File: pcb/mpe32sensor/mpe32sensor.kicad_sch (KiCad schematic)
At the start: 6 parts, among them J1 Conn_01x04, J2 Conn_01x01, J3 Conn_01x01, U1 TMAG5273

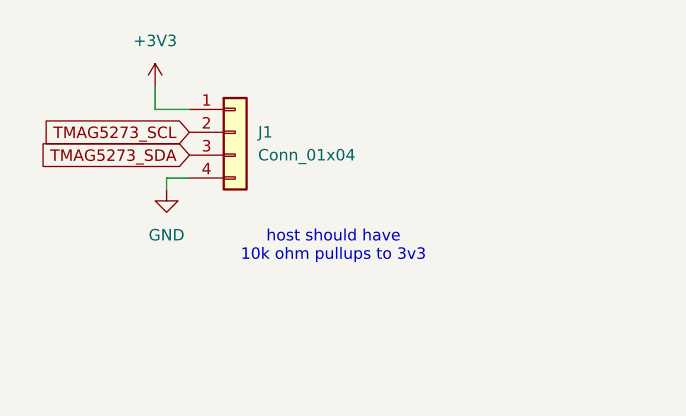
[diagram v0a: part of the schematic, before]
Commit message: production file changes + ide setup
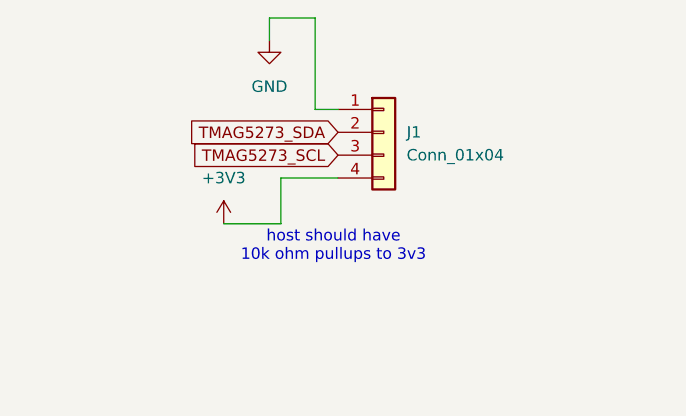
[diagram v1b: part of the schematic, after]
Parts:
- C1: MPN (none) -> 100nF 0603 X7R
- D1: MPN (none) -> SK6812MINI-E OPSCO Optoelectronics C5149201
- J1: MPN (none) -> SM04B-SRSS-TB
- J2, J3: MPN (none) -> DNP
- U1: MPN (none) -> TMAG5273A1
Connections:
- net +3V3: now also J1.4 (Pin_4); no longer J1.1 (Pin_1)
- net GND: now also J1.1 (Pin_1); no longer J1.4 (Pin_4)
- net TMAG5273_SCL: now also J1.3 (Pin_3); no longer J1.2 (Pin_2)
- net TMAG5273_SDA: now also J1.2 (Pin_2); no longer J1.3 (Pin_3)
